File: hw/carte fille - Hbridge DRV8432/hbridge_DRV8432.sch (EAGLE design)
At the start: 37 parts, among them IC1 DRV8402

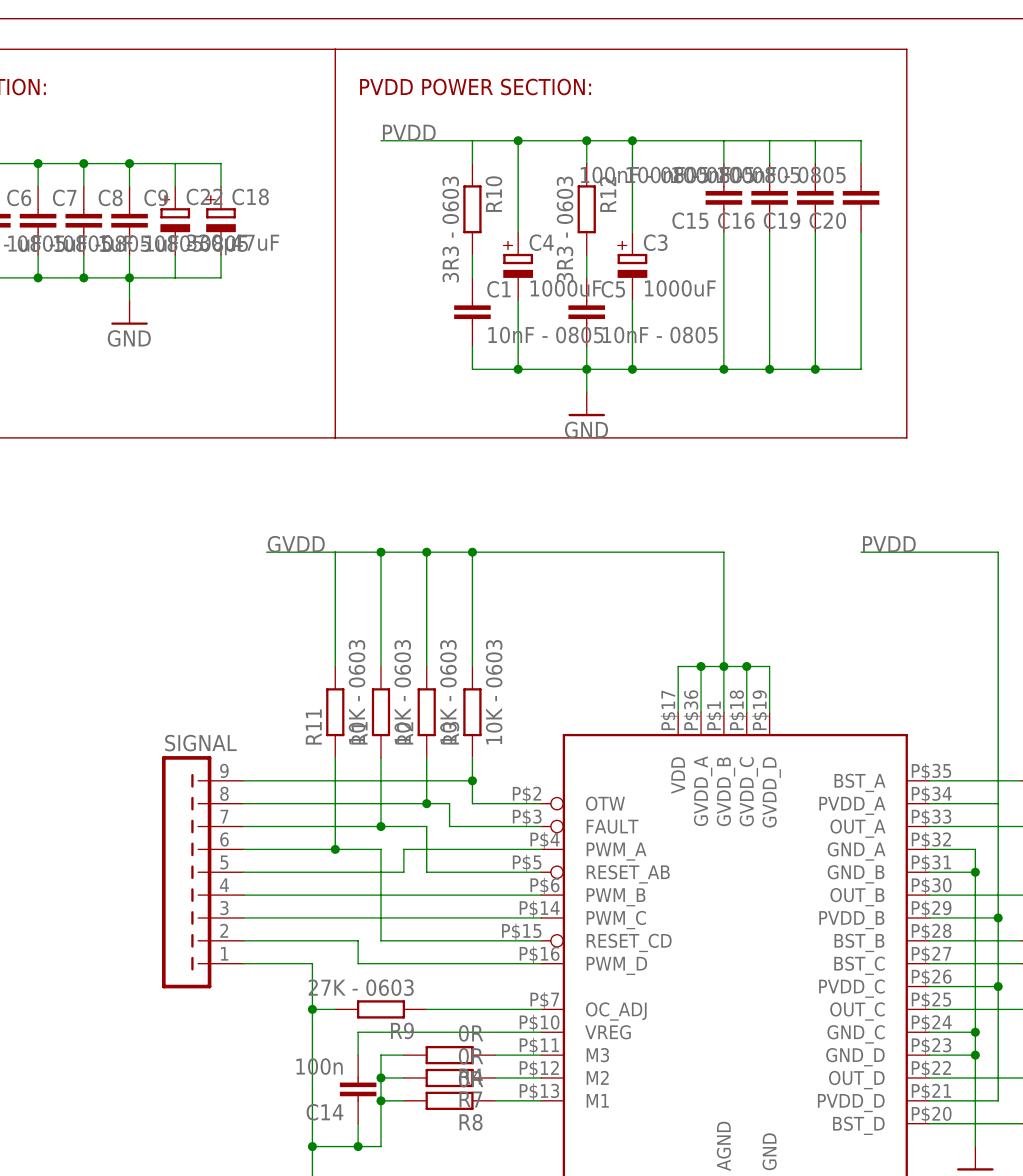
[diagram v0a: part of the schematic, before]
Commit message: Start routing the board
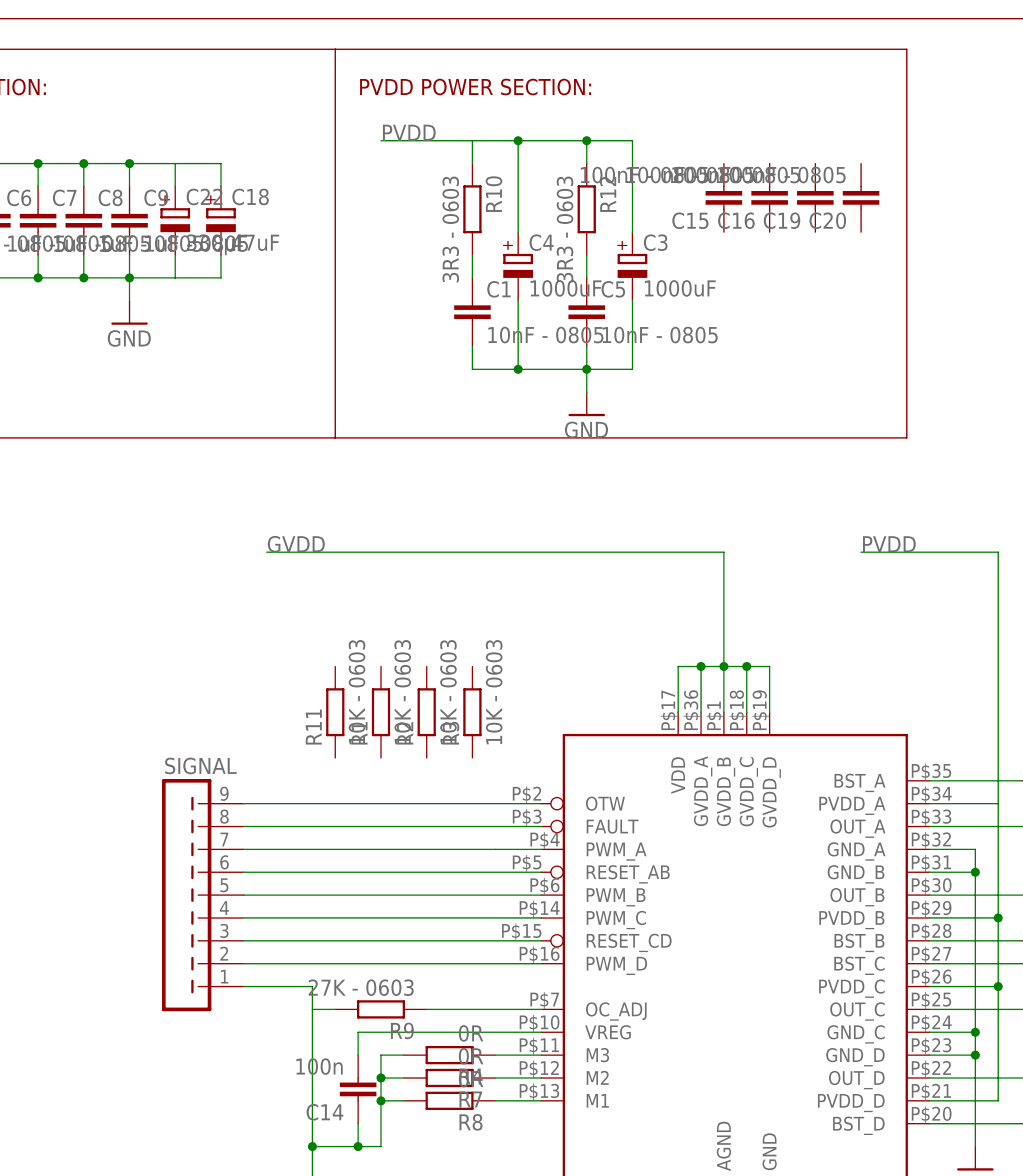
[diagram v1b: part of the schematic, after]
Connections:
- net GND: no longer C15.1, C16.1, C19.1, C20.1
- net GVDD: no longer R1.2, R11.2, R2.2, R3.2
- net N$1: no longer R3.1
- net N$16: now also IC1.RESET_AB; no longer IC1.RESET_CD, R11.1
- net N$17: now also IC1.PWM_B; no longer IC1.PWM_A
- net N$18: now also IC1.PWM_C; no longer IC1.PWM_B
- net N$19: now also IC1.RESET_CD; no longer IC1.PWM_C
- net N$6: no longer R2.1
- net N$8: now also IC1.PWM_A; no longer IC1.RESET_AB, R1.1
- net PVDD: no longer C15.2, C16.2, C19.2, C20.2
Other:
- moved on the sheet: SIGNAL

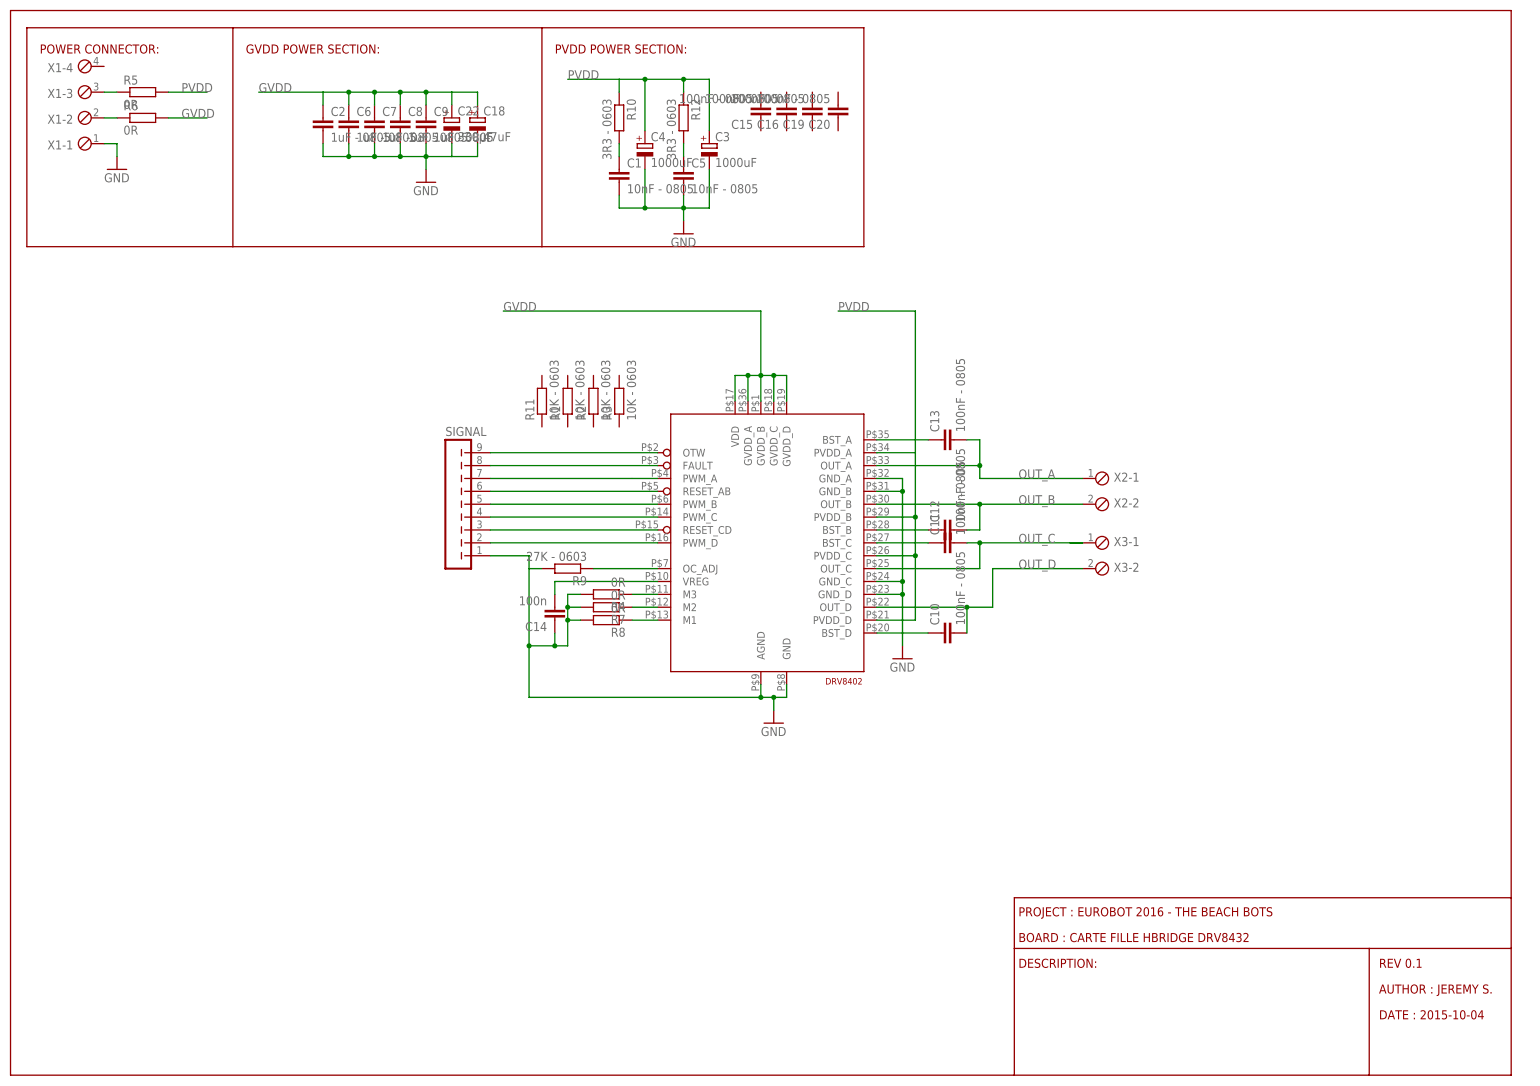
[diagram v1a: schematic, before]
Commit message: rework board routing
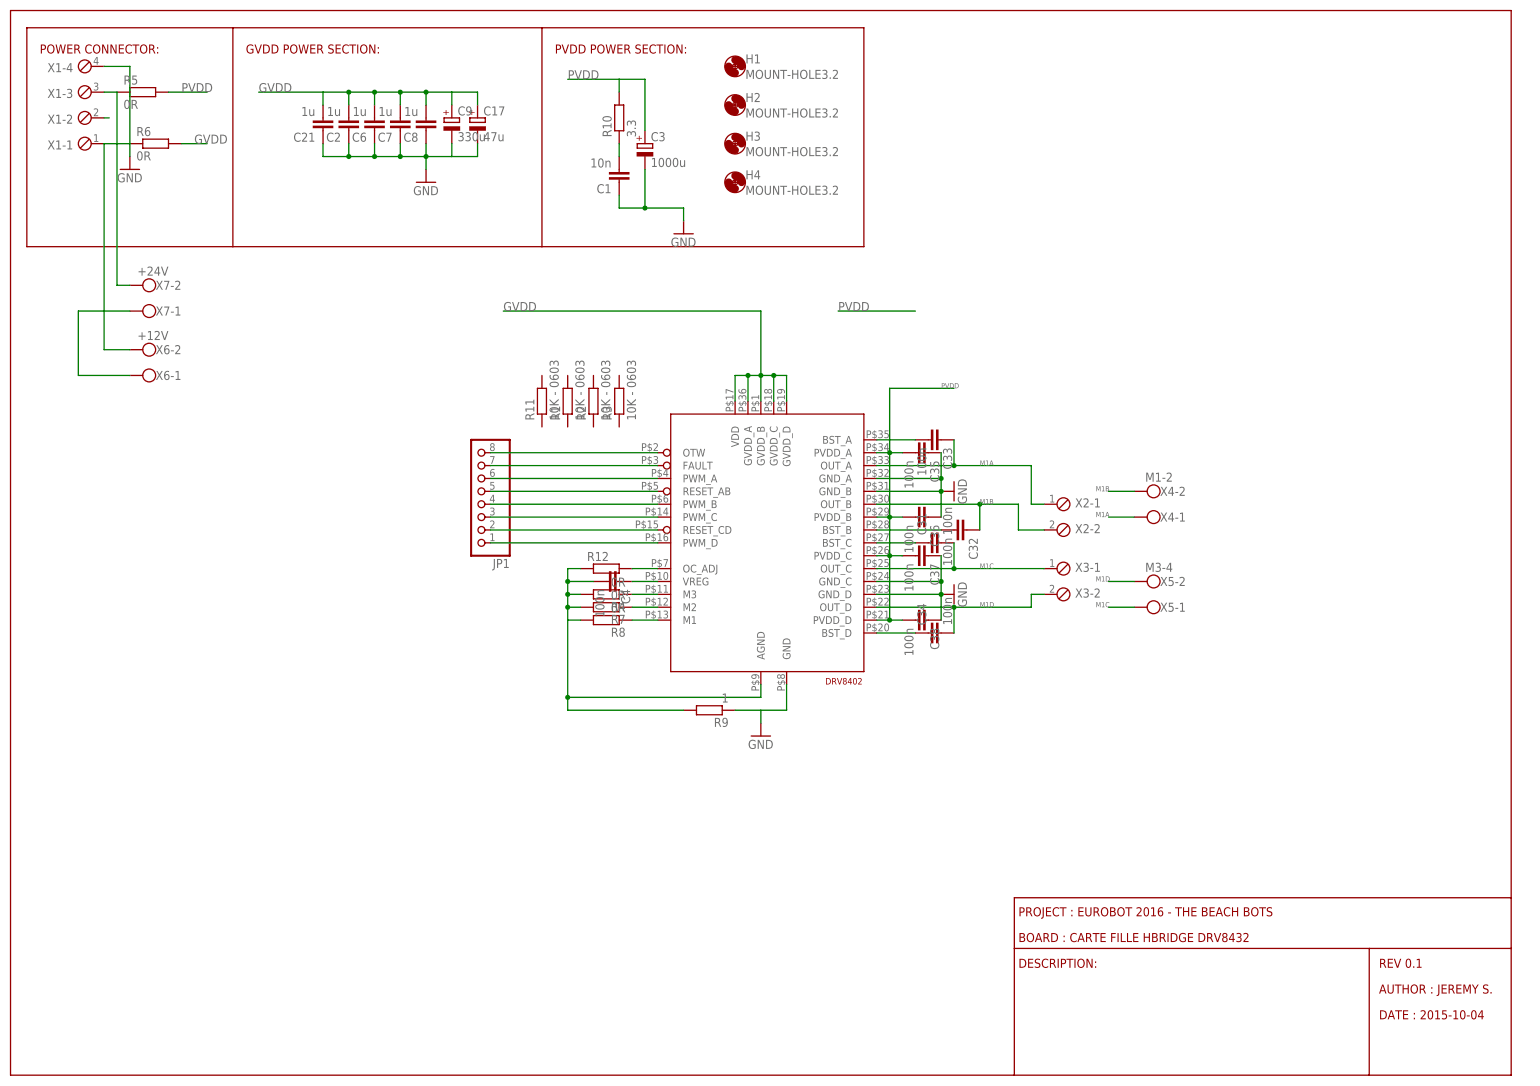
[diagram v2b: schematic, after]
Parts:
- removed C10, C11, C12, C13, C15, C16, C19, C20: 100nF - 0805, resistor:C-EUC0805
- removed C14: 100n, etienne:C_NP_805
- removed C18: 47uF, etienne:CPOL-EUE3.5-8
- removed C22: 330µF, etienne:CPOL-EUE3.5-8
- removed C5: 10nF - 0805, resistor:C-EUC0805
- removed SIGNAL: (no value), con-lsta:FE09-1
- added C17: 47u, rcl:CPOL-EUB/3528-21W
- added C21: 1u, rcl:C-EUC0805
- added C31, C32, C33, C34: 100n, rcl:C-EUC0805
- added C35, C36, C37, C38: 100n, rcl:C-EUC0603
- added H1, H2, H3, H4: MOUNT-HOLE3.2, holes:MOUNT-HOLE3.2
- added JP1: (no value), pinhead-2:PINHD-1X08_2.54
- added X4: M1-2, con-wago-500:W237-102
- added X5: M3-4, con-wago-500:W237-102
- added X6: +12V, con-wago-500:W237-102
- added X7: +24V, con-wago-500:W237-102
- C1: value 10nF - 0805 -> 10n; device resistor:C-EUC0805 -> rcl:C-EUC0805
- C2, C6, C8: value 1uF - 0805 -> 1u; device resistor:C-EUC0805 -> rcl:C-EUC0805
- C3: value 1000uF -> 1000u; device etienne:CPOL-EUE3.5-8 -> rcl:CPOL-EUE3.5-10
- C4: value 1000uF -> 100n; device etienne:CPOL-EUE3.5-8 -> rcl:C-EUC0603K
- C7: value 1uF -0805 -> 1u; device resistor:C-EUC0805 -> rcl:C-EUC0805
- C9: value 1uF - 0805 -> 330u; device resistor:C-EUC0805 -> rcl:CPOL-EUB/3528-21W
- R10: value 3R3 - 0603 -> 3.3; device resistor:R-EU_R0603 -> rcl:R-EU_R1206
- R12: value 3R3 - 0603 -> (none); device resistor:R-EU_R0603 -> rcl:R-EU_R0603
- R9: value 27K - 0603 -> 1; device resistor:R-EU_R0603 -> rcl:R-EU_R0603
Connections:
- removed net N$14: C5.1, R12.2
- removed net N$15: C13.1, IC1.BST_A
- removed net N$22: R5.1, X1-3.1
- removed net OUT_A: C13.2, IC1.OUT_A, X2-1.1
- removed net OUT_B: C12.2, IC1.OUT_B, X2-2.1
- removed net OUT_C: C11.2, IC1.OUT_C, X3-1.1
- removed net OUT_D: C10.2, IC1.OUT_D, X3-2.1
- new net GND1: X6-1.KL, X7-1.KL
- new net M1A: C33.1, IC1.OUT_A, X2-1.1, X4-1.KL
- new net M1B: C32.1, IC1.OUT_B, X2-2.1, X4-2.KL
- new net M1C: C31.2, IC1.OUT_C, X3-1.1, X5-1.KL
- new net M1D: C34.2, IC1.OUT_D, X3-2.1, X5-2.KL
- new net N$25: C33.2, IC1.BST_A
- new net N$26: C32.2, IC1.BST_B
- new net N$27: C31.1, IC1.BST_C
- new net N$28: C34.1, IC1.BST_D
- net GND: now also C1.1, C17.-, C2.1, C21.1, C35.1, C36.1, C37.1, C38.1, C6.1, C7.1, C8.1, C9.-, R9.1, X1-4.1; no longer C1.2, C14.1, C18.-, C2.2, C22.-, C4.-, C5.2, C6.2, C7.2, C8.2, C9.2, IC1.AGND, R4.2, R7.2, R8.2, R9.2, SIGNAL.1, X1-1.1
- net GVDD: now also C17.+, C2.2, C21.2, C6.2, C7.2, C8.2, C9.+; no longer C18.+, C2.1, C22.+, C6.1, C7.1, C8.1, C9.1
- net N$1: now also JP1.8; no longer SIGNAL.9
- net N$10: now also IC1.OC_ADJ, R12.2; no longer C12.1, IC1.BST_B
- net N$11: now also C4.1; no longer C14.2
- net N$12: now also X1-2.1; no longer C10.1, IC1.BST_D
- net N$13: now also C1.2, R10.1; no longer C1.1, R10.2
- net N$16: now also JP1.5; no longer SIGNAL.6
- net N$17: now also JP1.4; no longer SIGNAL.5
- net N$18: now also JP1.3; no longer SIGNAL.4
- net N$19: now also JP1.2; no longer SIGNAL.3
- net N$2: now also X1-1.1, X6-2.KL; no longer X1-2.1
- net N$20: now also JP1.1; no longer SIGNAL.2
- net N$6: now also JP1.7; no longer SIGNAL.8
- net N$7: now also R5.1, X1-3.1, X7-2.KL; no longer C11.1, IC1.BST_C
- net N$8: now also JP1.6; no longer SIGNAL.7
- net N$9: now also C4.2, IC1.AGND, R12.1, R4.2, R7.2, R8.2, R9.2; no longer IC1.OC_ADJ, R9.1
- net PVDD: now also C35.2, C36.2, C37.2, C38.2, R10.2; no longer C4.+, R10.1, R12.1
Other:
- moved on the sheet: C1, C2, C3, C6, C7, C8, R10, R12, R6, R9, X2-1, X2-2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
